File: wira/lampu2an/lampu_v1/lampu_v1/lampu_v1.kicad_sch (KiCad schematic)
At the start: 29 parts, among them J1 Conn_01x15_Pin, J10 FET, J11 Conn_01x03_Pin, J12 Conn_01x03_Pin, J13 Conn_01x03_Pin, J14 OUT1, J15 OUT2, J16 OUT3, J17 OUT4, J2 Conn_01x15_Pin, J3 Conn_01x15_Socket, J4 Conn_01x15_Socket, J5 Conn_01x15_Socket, J6 Conn_01x15_Socket, J7 Barrel_Jack_Switch, J8 Conn_01x02, J9 FAN, U1 NodeMCU1.0(ESP-12E), U2 L7805, U3 L7812

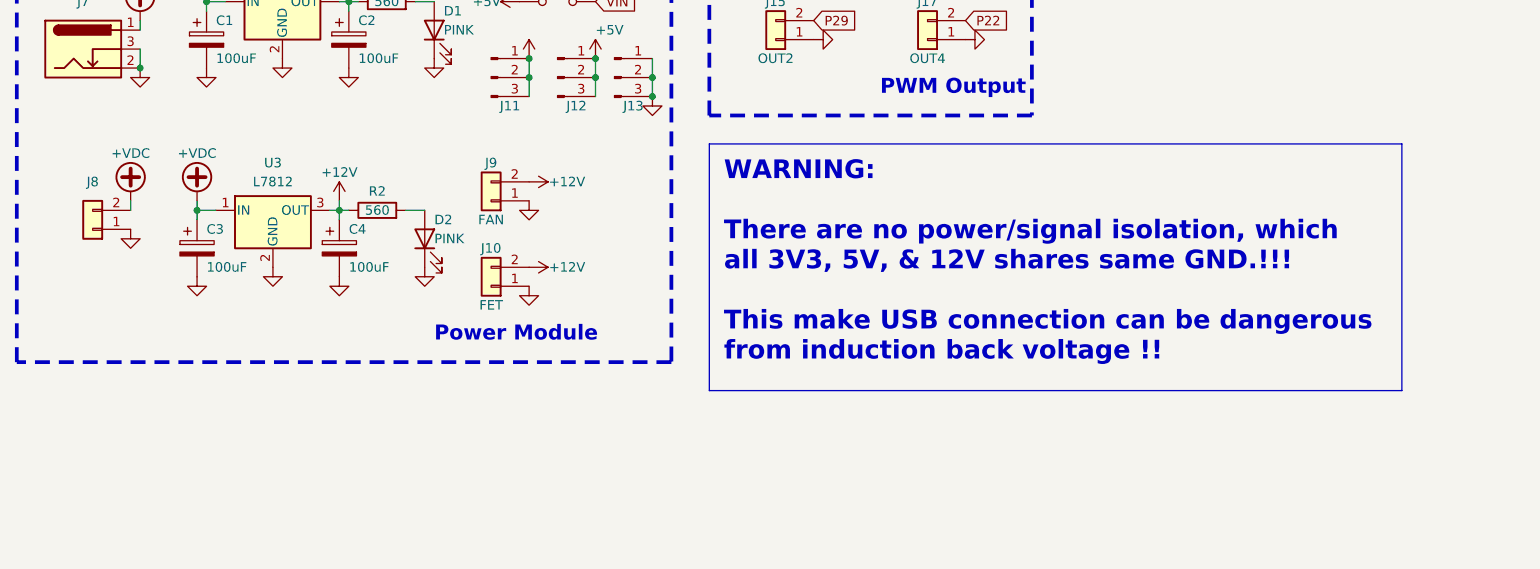
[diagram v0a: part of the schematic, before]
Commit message: Wira PCB
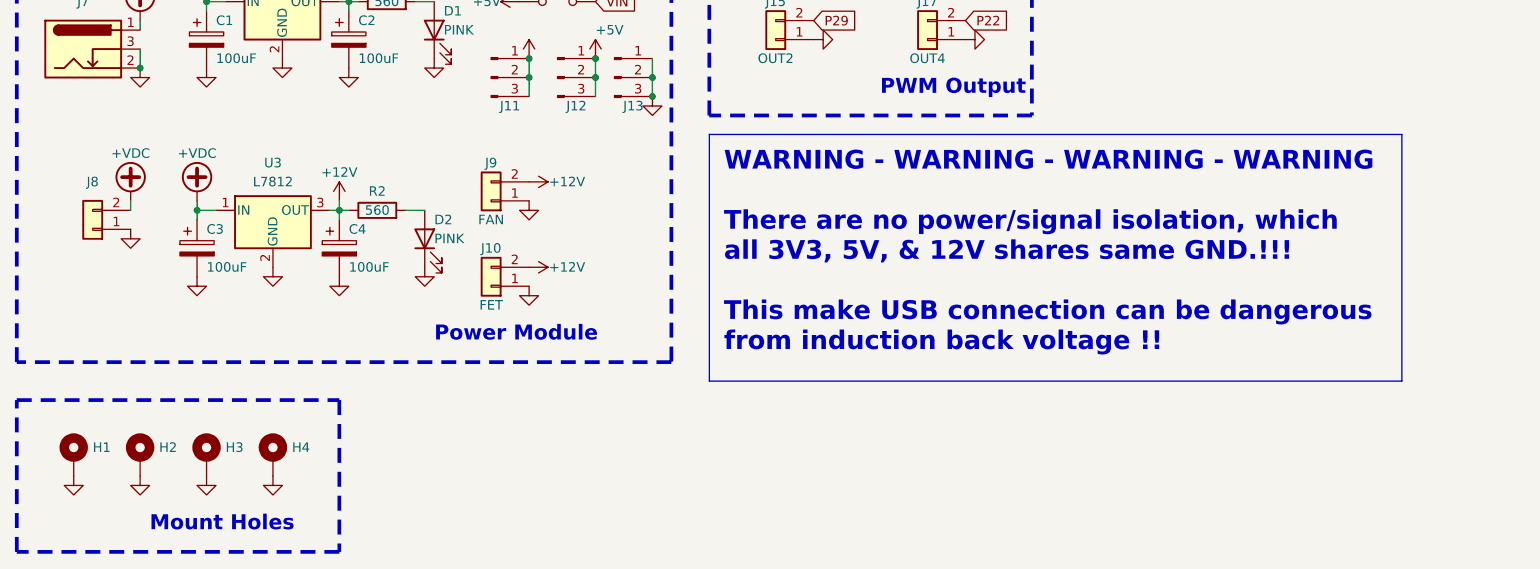
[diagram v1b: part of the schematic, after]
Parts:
- added H1, H2, H3, H4: MountingHole_Pad, symbol Mechanical:MountingHole_Pad
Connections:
- net GND: now also H1.1, H2.1, H3.1, H4.1
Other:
- note added: "Mount Holes"
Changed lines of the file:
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@@
+    (fill (type none))
+  )
+  (rectangle (start 27.94 153.67) (end 71.12 173.99)
+    (stroke (width 0.5) (type dash))
     (fill (type none))
   )
@@
     (fill (type none))
   )
-  (text_box "WARNING:\n\nThere are no power/signal isolation, which all 3V3, 5V, & 12V shares same GND.!!!\n\nThis make USB connection can be dangerous from induction back voltage !! "
-    (at 120.65 119.38 0) (size 92.71 33.02)
+  (text_box "WARNING - WARNING - WARNING - WARNING\n\nThere are no power/signal isolation, which all 3V3, 5V, & 12V shares same GND.!!!\n\nThis make USB connection can be dangerous from induction back voltage !! "
+    (at 120.65 118.11 0) (size 92.71 33.02)
     (stroke (width 0) (type default))
     (fill (type none))
@@
   )
   (text "NodeMCU Header Group" (at 153.67 80.01 0)
+    (effects (font (size 2 2) (thickness 0.4) bold) (justify left bottom))
+  )
+  (text "Mount Holes\n" (at 45.72 171.45 0)
     (effects (font (size 2 2) (thickness 0.4) bold) (justify left bottom))
   )
@@
         (path "/714d5fa9-02bc-42e1-ac93-ccd9a9b9e730"
           (reference "#PWR051") (unit 1)
+        )
+      )
+    )
+  )
+  (symbol (lib_id "power:GND") (at 53.34 163.83 0) (unit 1)
+    (in_bom yes) (on_board yes) (dnp no) (fields_autoplaced)
+    (property "Reference" "#PWR059" (at 53.34 170.18 0)
+      (effects (font (size 1.27 1.27)) hide)
+    )
+    (property "Value" "GND" (at 53.34 167.64 90)
+      (effects (font (size 1.27 1.27)) (justify right) hide)
+    )
+    (property "Footprint" "" (at 53.34 163.83 0)
+      (effects (font (size 1.27 1.27)) hide)
+    )
+    (property "Datasheet" "" (at 53.34 163.83 0)
+      (effects (font (size 1.27 1.27)) hide)
+    )
+    (pin "1")
+    (instances
+      (project "lampu_v1"
+        (path "/714d5fa9-02bc-42e1-ac93-ccd9a9b9e730"
+          (reference "#PWR059") (unit 1)
         )
       )
@@
     )
   )
+  (symbol (lib_id "Mechanical:MountingHole_Pad") (at 44.45 161.29 0) (unit 1)
+    (in_bom yes) (on_board yes) (dnp no) (fields_autoplaced)
+    (property "Reference" "H2" (at 46.99 160.02 0)
+      (effects (font (size 1.27 1.27)) (justify left))
+    )
+    (property "Value" "MountingHole_Pad" (at 46.99 161.29 0)
+      (effects (font (size 1.27 1.27)) (justify left) hide)
+    )
+    (property "Footprint" "" (at 44.45 161.29 0)
+      (effects (font (size 1.27 1.27)) hide)
+    )
+    (property "Datasheet" "~" (at 44.45 161.29 0)
+      (effects (font (size 1.27 1.27)) hide)
+    )
+    (pin "1")
+    (instances
+      (project "lampu_v1"
+        (path "/714d5fa9-02bc-42e1-ac93-ccd9a9b9e730"
+          (reference "H2") (unit 1)
+        )
+      )
+    )
+  )
   (symbol (lib_id "power:VDD") (at 151.13 38.1 270) (mirror x) (unit 1)
     (in_bom yes) (on_board yes) (dnp no) (fields_autoplaced)
@@
         (path "/714d5fa9-02bc-42e1-ac93-ccd9a9b9e730"
           (reference "#PWR019") (unit 1)
+        )
+      )
+    )
+  )
+  (symbol (lib_id "Mechanical:MountingHole_Pad") (at 62.23 161.29 0) (unit 1)
+    (in_bom yes) (on_board yes) (dnp no) (fields_autoplaced)
+    (property "Reference" "H4" (at 64.77 160.02 0)
+      (effects (font (size 1.27 1.27)) (justify left))
+    )
+    (property "Value" "MountingHole_Pad" (at 64.77 161.29 0)
+      (effects (font (size 1.27 1.27)) (justify left) hide)
+    )
+    (property "Footprint" "" (at 62.23 161.29 0)
+      (effects (font (size 1.27 1.27)) hide)
+    )
+    (property "Datasheet" "~" (at 62.23 161.29 0)
+      (effects (font (size 1.27 1.27)) hide)
+    )
+    (pin "1")
+    (instances
+      (project "lampu_v1"
+        (path "/714d5fa9-02bc-42e1-ac93-ccd9a9b9e730"
+          (reference "H4") (unit 1)
+        )
+      )
+    )
+  )
+  (symbol (lib_id "power:GND") (at 44.45 163.83 0) (unit 1)
+    (in_bom yes) (on_board yes) (dnp no) (fields_autoplaced)
+    (property "Reference" "#PWR058" (at 44.45 170.18 0)
+      (effects (font (size 1.27 1.27)) hide)
+    )
+    (property "Value" "GND" (at 44.45 167.64 90)
+      (effects (font (size 1.27 1.27)) (justify right) hide)
+    )
+    (property "Footprint" "" (at 44.45 163.83 0)
+      (effects (font (size 1.27 1.27)) hide)
+    )
+    (property "Datasheet" "" (at 44.45 163.83 0)
+      (effects (font (size 1.27 1.27)) hide)
+    )
+    (pin "1")
+    (instances
+      (project "lampu_v1"
+        (path "/714d5fa9-02bc-42e1-ac93-ccd9a9b9e730"
+          (reference "#PWR058") (unit 1)
         )
       )
@@
     )
   )
+  (symbol (lib_id "power:GND") (at 62.23 163.83 0) (unit 1)
+    (in_bom yes) (on_board yes) (dnp no) (fields_autoplaced)
+    (property "Reference" "#PWR060" (at 62.23 170.18 0)
+      (effects (font (size 1.27 1.27)) hide)
+    )
+    (property "Value" "GND" (at 62.23 167.64 90)
+      (effects (font (size 1.27 1.27)) (justify right) hide)
+    )
+    (property "Footprint" "" (at 62.23 163.83 0)
+      (effects (font (size 1.27 1.27)) hide)
+    )
+    (property "Datasheet" "" (at 62.23 163.83 0)
+      (effects (font (size 1.27 1.27)) hide)
+    )
+    (pin "1")
+    (instances
+      (project "lampu_v1"
+        (path "/714d5fa9-02bc-42e1-ac93-ccd9a9b9e730"
+          (reference "#PWR060") (unit 1)
+        )
+      )
+    )
+  )
   (symbol (lib_id "power:VDD") (at 166.37 63.5 270) (mirror x) (unit 1)
     (in_bom yes) (on_board yes) (dnp no) (fields_autoplaced)
@@
         (path "/714d5fa9-02bc-42e1-ac93-ccd9a9b9e730"
           (reference "#PWR043") (unit 1)
+        )
+      )
+    )
+  )
+  (symbol (lib_id "Mechanical:MountingHole_Pad") (at 35.56 161.29 0) (unit 1)
+    (in_bom yes) (on_board yes) (dnp no) (fields_autoplaced)
+    (property "Reference" "H1" (at 38.1 160.02 0)
+      (effects (font (size 1.27 1.27)) (justify left))
+    )
+    (property "Value" "MountingHole_Pad" (at 38.1 161.29 0)
+      (effects (font (size 1.27 1.27)) (justify left) hide)
+    )
+    (property "Footprint" "" (at 35.56 161.29 0)
+      (effects (font (size 1.27 1.27)) hide)
+    )
+    (property "Datasheet" "~" (at 35.56 161.29 0)
+      (effects (font (size 1.27 1.27)) hide)
+    )
+    (pin "1")
+    (instances
+      (project "lampu_v1"
+        (path "/714d5fa9-02bc-42e1-ac93-ccd9a9b9e730"
+          (reference "H1") (unit 1)
         )
       )
@@
     )
   )
+  (symbol (lib_id "Mechanical:MountingHole_Pad") (at 53.34 161.29 0) (unit 1)
+    (in_bom yes) (on_board yes) (dnp no) (fields_autoplaced)
+    (property "Reference" "H3" (at 55.88 160.02 0)
+      (effects (font (size 1.27 1.27)) (justify left))
+    )
+    (property "Value" "MountingHole_Pad" (at 55.88 161.29 0)
+      (effects (font (size 1.27 1.27)) (justify left) hide)
+    )
+    (property "Footprint" "" (at 53.34 161.29 0)
+      (effects (font (size 1.27 1.27)) hide)
+    )
+    (property "Datasheet" "~" (at 53.34 161.29 0)
+      (effects (font (size 1.27 1.27)) hide)
+    )
+    (pin "1")
+    (instances
+      (project "lampu_v1"
+        (path "/714d5fa9-02bc-42e1-ac93-ccd9a9b9e730"
+          (reference "H3") (unit 1)
+        )
+      )
+    )
+  )
   (symbol (lib_id "Device:C_Polarized") (at 71.12 133.35 0) (unit 1)
     (in_bom yes) (on_board yes) (dnp no)
@@
         )
       )
+    )
+  )
+  (symbol (lib_id "power:GND") (at 35.56 163.83 0) (unit 1)
+    (in_bom yes) (on_board yes) (dnp no) (fields_autoplaced)
+    (property "Reference" "#PWR057" (at 35.56 170.18 0)
+      (effects (font (size 1.27 1.27)) hide)
+    )
+    (property "Value" "GND" (at 35.56 167.64 90)
+      (effects (font (size 1.27 1.27)) (justify right) hide)
+    )
+    (property "Footprint" "" (at 35.56 163.83 0)
+      (effects (font (size 1.27 1.27)) hide)
+    )
+    (property "Datasheet" "" (at 35.56 163.83 0)
+      (effects (font (size 1.27 1.27)) hide)
+    )
+    (pin "1")
+    (instances
+      (project "lampu_v1"
+        (path "/714d5fa9-02bc-42e1-ac93-ccd9a9b9e730"
+          (reference "#PWR057") (unit 1)
+        )
+      )

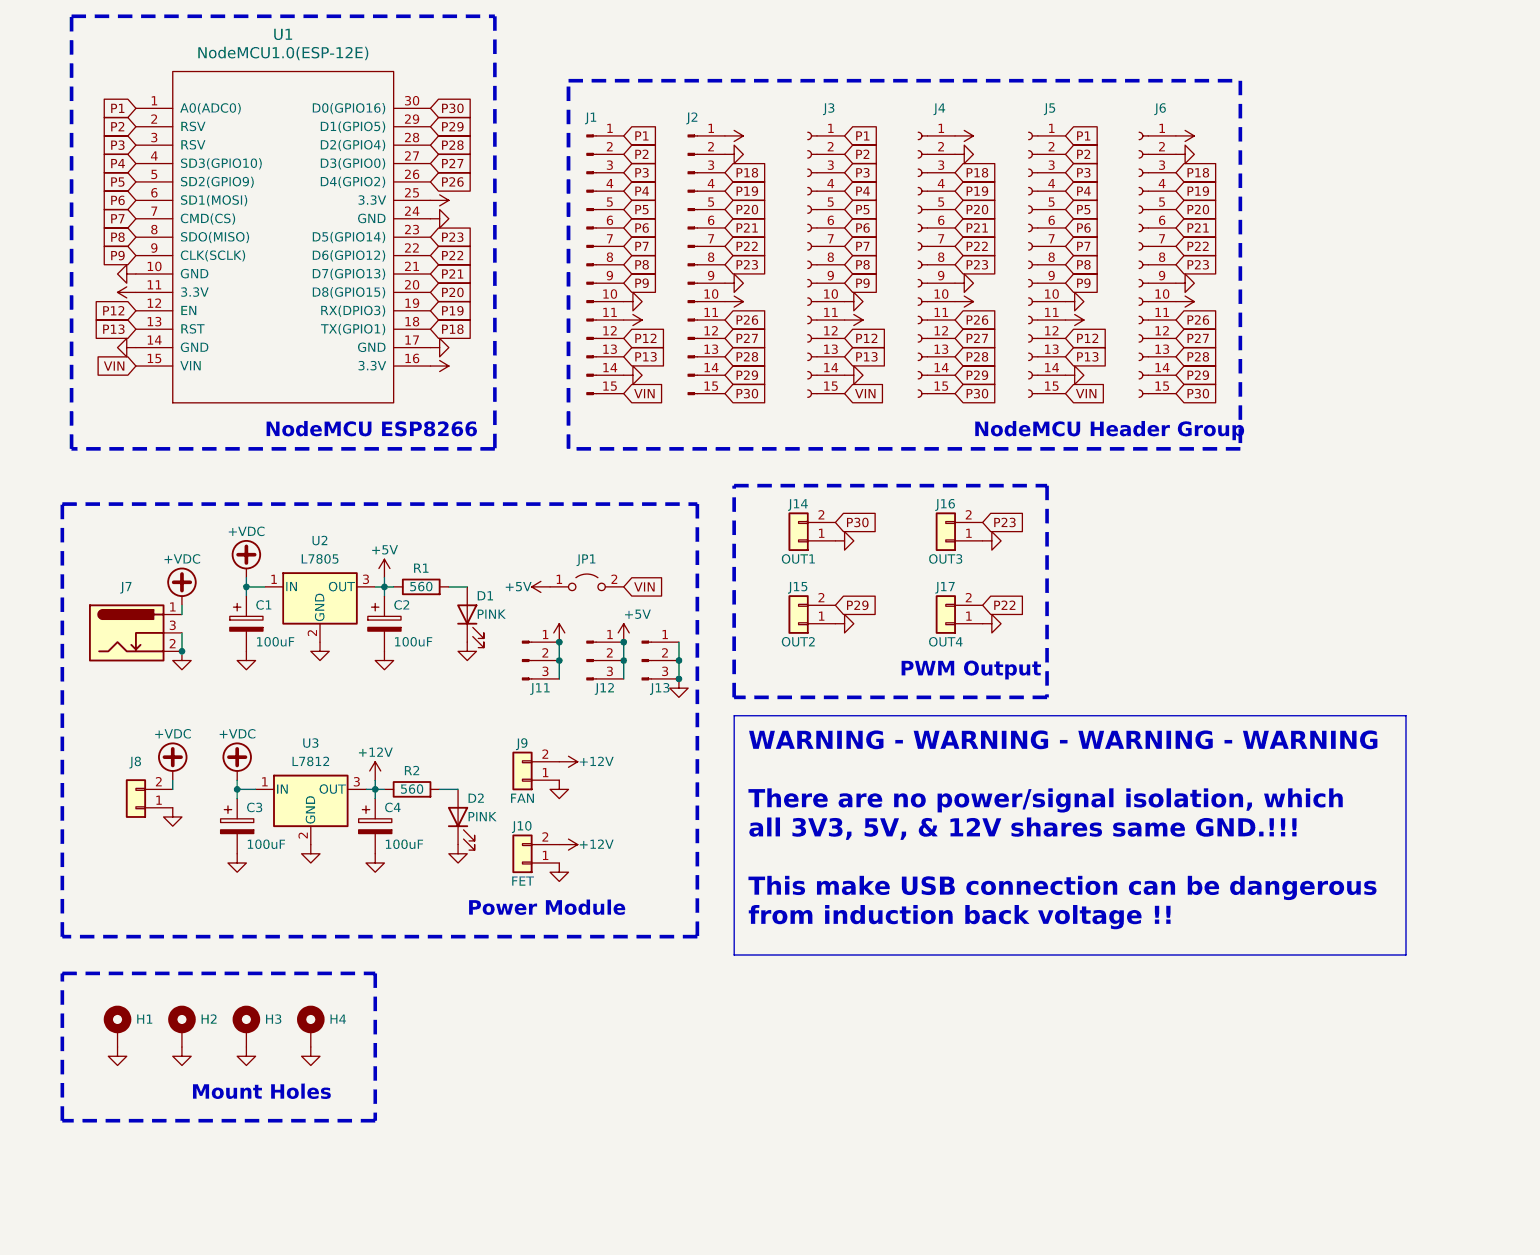
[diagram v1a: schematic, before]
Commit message: Lampunya Wira
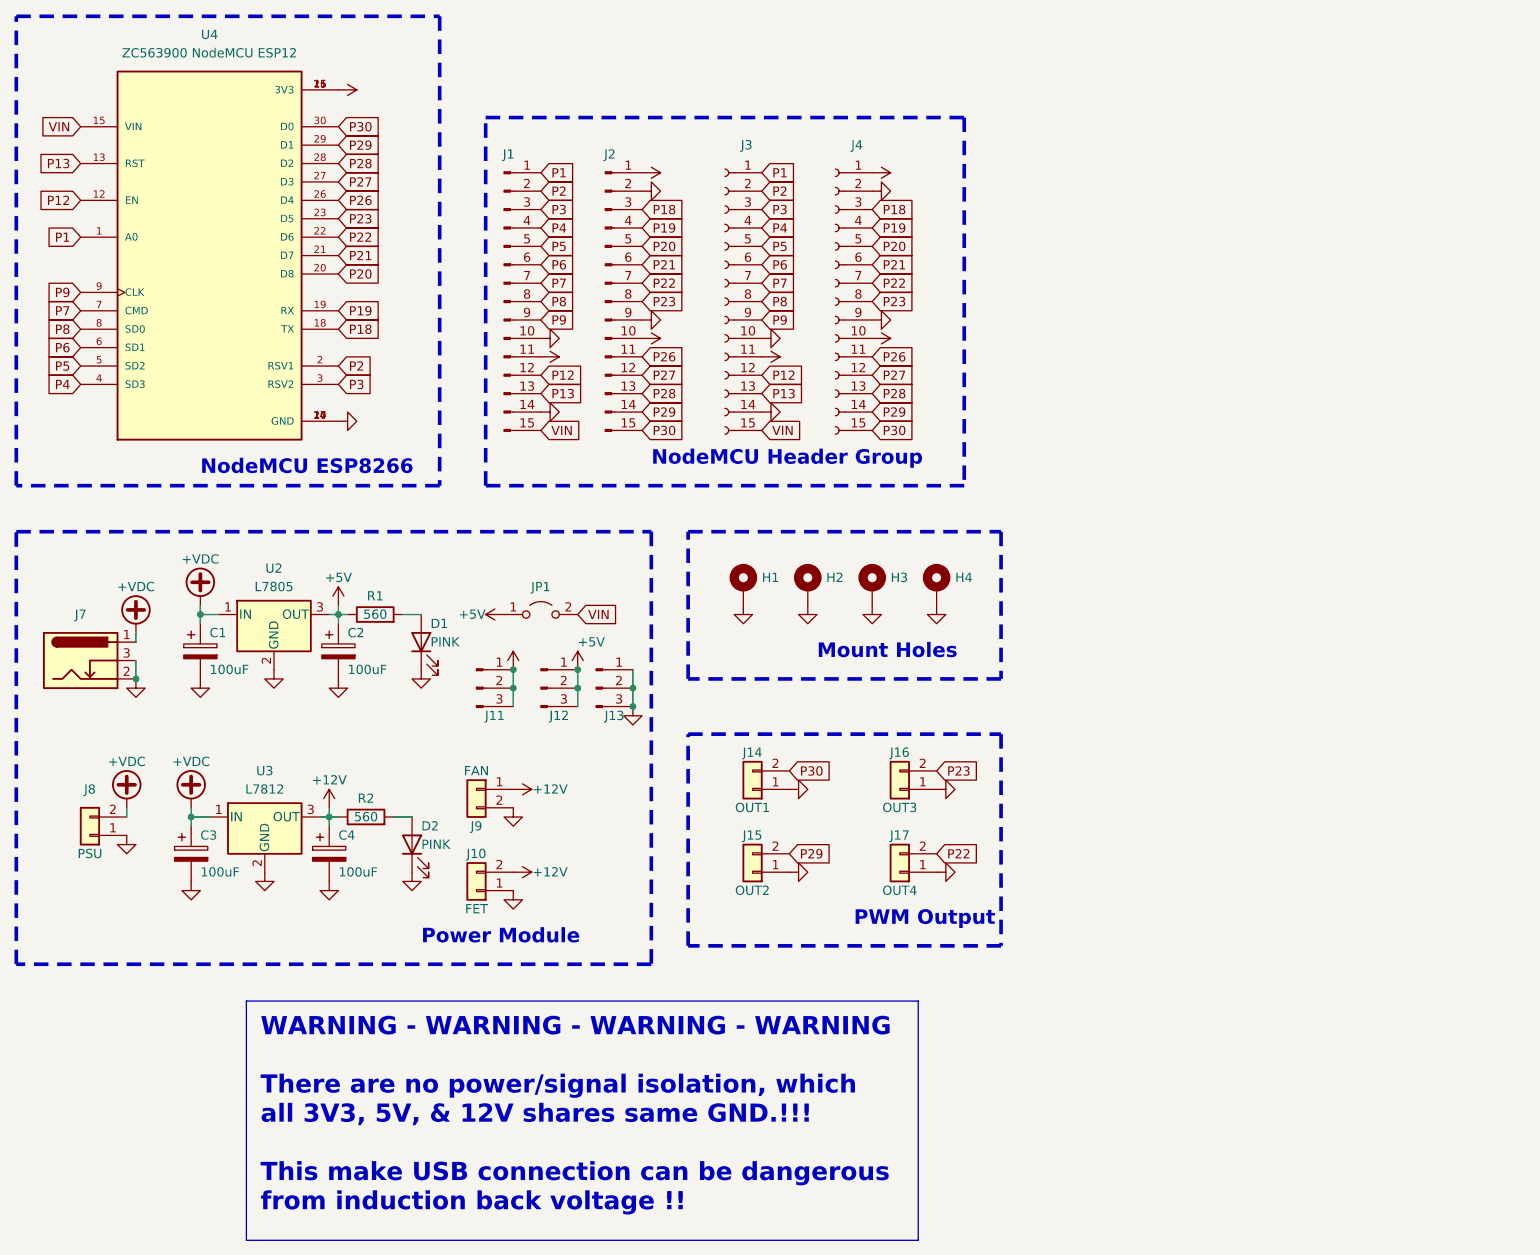
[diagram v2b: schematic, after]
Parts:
- removed J5, J6: Conn_01x15_Socket, symbol Connector:Conn_01x15_Socket
- removed U1: NodeMCU1.0(ESP-12E), symbol ESP8266:NodeMCU1.0(ESP-12E)
- added U4: ZC563900 NodeMCU ESP12, NodeMCU:MODULE_ZC563900, symbol ZC563900:ZC563900
- C1, C2, C3, C4: footprint (none) -> Capacitor_THT:CP_Radial_D5.0mm_P2.50mm
- D1, D2: footprint (none) -> LED_THT:LED_D3.0mm
- H1, H2, H3, H4: footprint (none) -> MountingHole:MountingHole_2.5mm_Pad
- J1, J2: footprint (none) -> Connector_PinHeader_2.54mm:PinHeader_1x15_P2.54mm_Vertical
- J10, J14, J15, J16, J17: footprint (none) -> TerminalBlock:TerminalBlock_Altech_AK300-2_P5.00mm
- J11, J12, J13: footprint (none) -> Connector_PinHeader_2.54mm:PinHeader_1x03_P2.54mm_Vertical
- J3, J4: footprint (none) -> Connector_PinSocket_2.54mm:PinSocket_1x15_P2.54mm_Vertical
- J7: footprint (none) -> Connector_BarrelJack:BarrelJack_Horizontal
- J8: value Conn_01x02 -> PSU; footprint (none) -> TerminalBlock:TerminalBlock_Altech_AK300-2_P5.00mm
- J9: footprint (none) -> Connector_JST:JST_XH_B2B-XH-A_1x02_P2.50mm_Vertical
- JP1: footprint (none) -> Jumper:SolderJumper-2_P1.3mm_Open_RoundedPad1.0x1.5mm
- R1, R2: footprint (none) -> Resistor_THT:R_Axial_DIN0207_L6.3mm_D2.5mm_P7.62mm_Horizontal
- U2, U3: footprint (none) -> Package_TO_SOT_THT:TO-220F-3_Vertical
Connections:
- net +12V: now also J9.1 (Pin_1); no longer J9.2 (Pin_2)
- net GND: now also J9.2 (Pin_2), U4.10 (GND), U4.14 (GND), U4.17 (GND), U4.24 (GND); no longer J9.1 (Pin_1)
- net P1: now also U4.1 (A0)
- net P12: now also U4.12 (EN)
- net P13: now also U4.13 (RST)
- net P18: now also U4.18 (TX)
- net P19: now also U4.19 (RX)
- net P2: now also U4.2 (RSV1)
- net P20: now also U4.20 (D8)
- net P21: now also U4.21 (D7)
- net P22: now also U4.22 (D6)
- net P23: now also U4.23 (D5)
- net P26: now also U4.26 (D4)
- net P27: now also U4.27 (D3)
- net P28: now also U4.28 (D2)
- net P29: now also U4.29 (D1)
- net P3: now also U4.3 (RSV2)
- net P30: now also U4.30 (D0)
- net P4: now also U4.4 (SD3)
- net P5: now also U4.5 (SD2)
- net P6: now also U4.6 (SD1)
- net P7: now also U4.7 (CMD)
- net P8: now also U4.8 (SD0)
- net P9: now also U4.9 (CLK)
- net VDD: now also U4.11 (3V3), U4.16 (3V3), U4.25 (3V3)
- net VIN: now also U4.15 (VIN)
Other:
- moved on the sheet: C1, C2, C3, C4, D1, D2, H1, H2, H3, H4, J1, J10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
